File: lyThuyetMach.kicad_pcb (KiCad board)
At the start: 2 copper layers, 48 x 79 mm, 34 parts, among them J1 USB_C_Receptacle_PowerOnly_6P, J2 Voltage_Booster, J4 Out_LED, Q1 BC547, Q2 BC547, Q3 BC547, Q4 BC547, Q5 BC547, Q6 BC547, Q7 TIP122, SW1 SW_SPDT, SW2 SW_SPDT

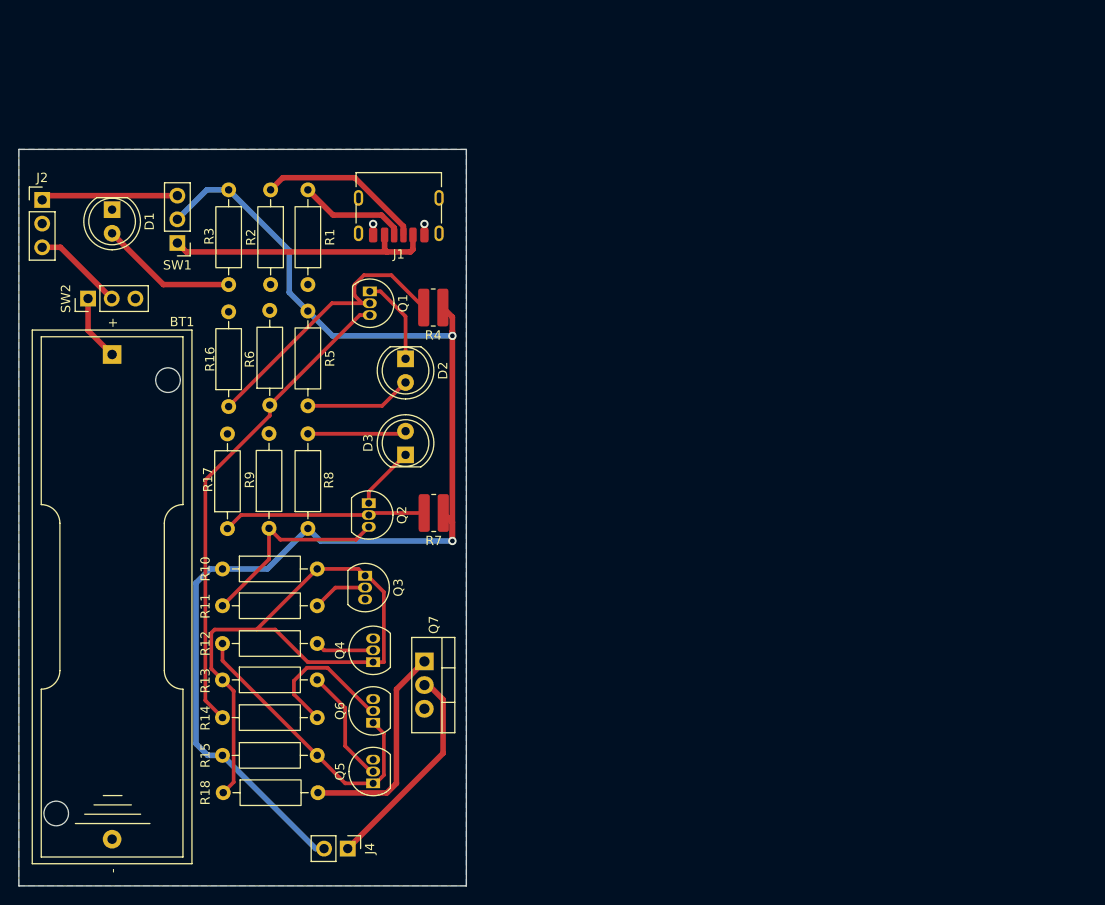
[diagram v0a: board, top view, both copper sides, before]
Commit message: Add files via upload
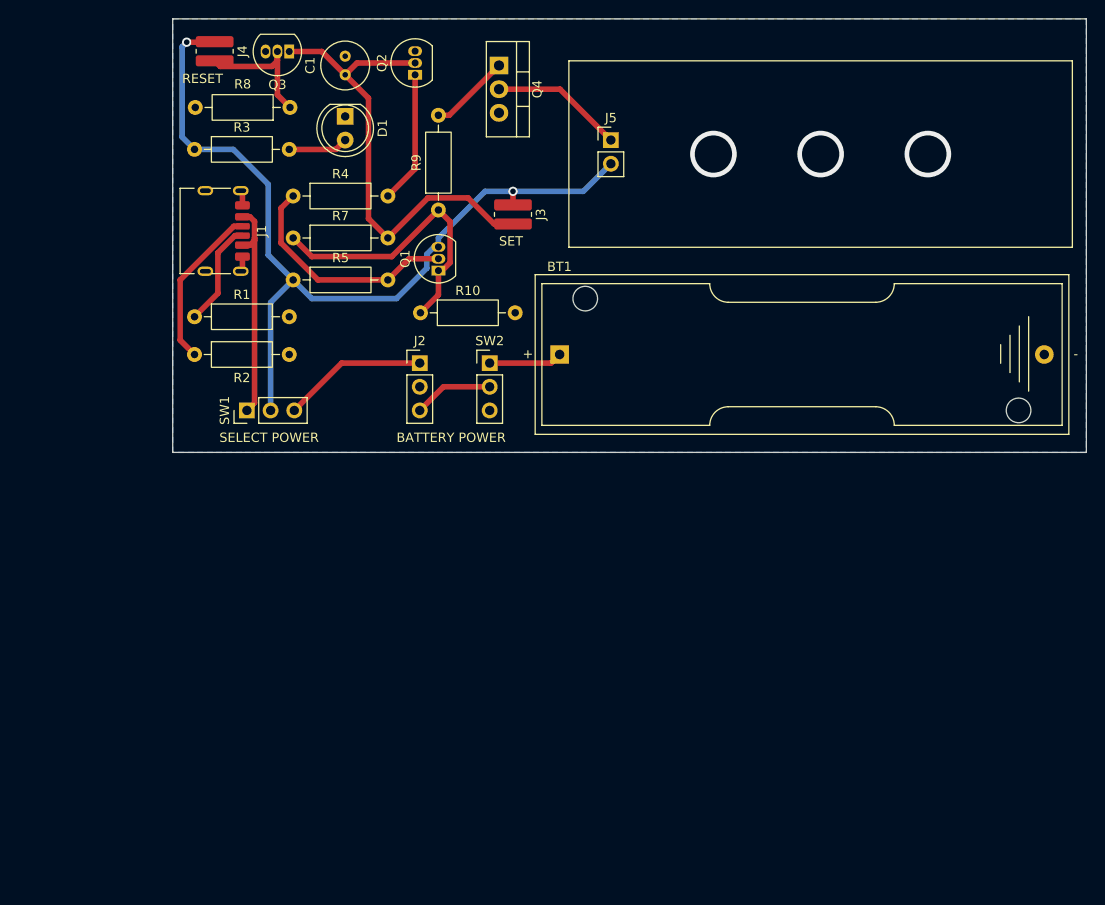
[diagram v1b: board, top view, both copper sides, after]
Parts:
- removed D2, D3: LED, LED_THT:LED_D5.0mm_FlatTop
- removed Q5, Q6: BC547, Package_TO_SOT_THT:TO-92_Inline
- removed Q7: TIP122, Package_TO_SOT_THT:TO-220-3_Vertical
- removed R11, R12, R13, R14, R18: 1k, Resistor_THT:R_Axial_DIN0207_L6.3mm_D2.5mm_P10.16mm_Horizontal
- removed R15: 470, Resistor_THT:R_Axial_DIN0207_L6.3mm_D2.5mm_P10.16mm_Horizontal
- removed R16, R17: 1M, Resistor_THT:R_Axial_DIN0207_L6.3mm_D2.5mm_P10.16mm_Horizontal
- removed R6: 4.7k, Resistor_THT:R_Axial_DIN0207_L6.3mm_D2.5mm_P10.16mm_Horizontal
- added C1: 100n, Capacitor_THT:C_Radial_D5.0mm_H5.0mm_P2.00mm, F.Cu at (89.5, 37.0)
- added J3: Conn_01x02_Pin, Resistor_SMD:R_0815_2038Metric_Pad1.20x4.05mm_HandSolder, F.Cu at (107.5, 52.0)
- added J5: Out_LED, Connector_PinHeader_2.54mm:PinHeader_1x02_P2.54mm_Vertical, F.Cu at (118.0, 44.0)
- J4: value Out_LED -> Conn_01x02_Pin; footprint Connector_PinHeader_2.54mm:PinHeader_1x02_P2.54mm_Vertical -> Resistor_SMD:R_0815_2038Metric_Pad1.20x4.05mm_HandSolder
- Q1: value BC547 -> BC557
- Q4: value BC547 -> TIP122; footprint Package_TO_SOT_THT:TO-92_Inline -> Package_TO_SOT_THT:TO-220-3_Vertical
- R10: value 470 -> 10k
- R4: value 0 -> 4.7k; footprint Resistor_SMD:R_0815_2038Metric_Pad1.20x4.05mm_HandSolder -> Resistor_THT:R_Axial_DIN0207_L6.3mm_D2.5mm_P10.16mm_Horizontal
- R5: value 100 -> 4.7k
- R7: value 0 -> 10k; footprint Resistor_SMD:R_0815_2038Metric_Pad1.20x4.05mm_HandSolder -> Resistor_THT:R_Axial_DIN0207_L6.3mm_D2.5mm_P10.16mm_Horizontal
- R8: value 100 -> 1M
- R9: value 4.7k -> 1k
- moved J4 86.7 mm to (75.5, 34.5)
- moved Q4 65.4 mm to (106.0, 36.0), turned to -90 degrees
- moved Q3 56.8 mm to (83.5, 34.5), turned to 180 degrees
- moved BT1 48.0 mm to (112.5, 67.0), turned to 0 degrees
- moved Q2 46.2 mm to (97.0, 37.0), turned to 90 degrees
- moved R8 45.2 mm to (83.6, 40.5), turned to 180 degrees
- moved J2 44.1 mm to (97.5, 67.9)
- moved SW2 43.6 mm to (105.0, 67.9), turned to 0 degrees
- moved R9 38.7 mm to (99.5, 51.5)
- moved R10 34.7 mm to (97.6, 62.5)
- moved R7 33.1 mm to (83.9, 54.5), turned to 0 degrees
- moved D1 26.9 mm to (89.5, 41.5)
- moved J1 20.1 mm to (75.3, 53.8), turned to -90 degrees
- moved R2 19.5 mm to (73.3, 67.0), turned to 0 degrees
- moved SW1 19.4 mm to (79.0, 73.0), turned to 90 degrees
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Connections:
- J4 pad 1: Net-(J4-Pin_1) -> VCC
- J4 pad 2: VCC -> Net-(J4-Pin_2)
- Q1 pad 1: Net-(D2-K) -> /LED TOGGLE
- Q1 pad 3: SET -> VCC
- Q2 pad 1: Net-(D3-K) -> Net-(Q2-C)
- Q2 pad 2: Net-(Q2-B) -> Net-(J3-Pin_2)
- Q2 pad 3: RESET -> USB_GND
- Q3 pad 1: LED_Toggle -> Net-(J3-Pin_2)
- Q3 pad 2: Net-(Q3-B) -> Net-(J4-Pin_2)
- Q4 pad 1: LED_Toggle -> Net-(Q4-B)
- Q4 pad 2: Net-(Q4-B) -> /OUT_LED_NE
- R10 pad 1: VCC -> /LED TOGGLE
- R10 pad 2: LED_Toggle -> USB_GND
- R4 pad 1: VCC -> Net-(Q1-B)
- R4 pad 2: Net-(Q1-B) -> Net-(Q2-C)
- R5 pad 2: Net-(D2-A) -> Net-(Q1-B)
- R7 pad 1: VCC -> /LED TOGGLE
- R7 pad 2: Net-(Q2-B) -> Net-(J3-Pin_2)
- R8 pad 1: VCC -> Net-(J4-Pin_2)
- R8 pad 2: Net-(D3-A) -> USB_GND
- R9 pad 1: RESET -> /LED TOGGLE
- R9 pad 2: USB_GND -> Net-(Q4-B)
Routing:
- net LED_Toggle: track 63.6 -> 0.00 mm
- net SET: track 51.9 -> 0.00 mm
- net Net-(J3-Pin_2): track 0.00 -> 50.8 mm
- net VCC: track 135.4 -> 94.9 mm
- net /LED TOGGLE: track 0.00 -> 31.6 mm
- net NOT_LED_Toggle: track 31.1 -> 0.00 mm
- net Net-(Q7-B): track 23.2 -> 0.00 mm
- net Net-(J4-Pin_1): track 22.9 -> 0.00 mm
- net RESET: track 22.1 -> 0.00 mm
- net Net-(Q2-B): track 21.8 -> 0.00 mm
- net Net-(Q6-B): track 16.0 -> 0.00 mm
- net Net-(J4-Pin_2): track 0.00 -> 14.8 mm
- net /OUT_LED_NE: track 0.00 -> 14.3 mm
- net Net-(Q2-C): track 0.00 -> 14.2 mm
- net Net-(Q5-B): track 12.5 -> 0.00 mm
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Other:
- board size 48 x 79 mm -> 98 x 46.5 mm
- board text added: "BATTERY POWER"
- board text added: "RESET"
- board text added: "SELECT POWER"
- board text added: "SET"
